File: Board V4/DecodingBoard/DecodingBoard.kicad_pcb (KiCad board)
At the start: 4 copper layers, 0 parts

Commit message: First version of the layout
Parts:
- added C1: 10 μF 6.3V X5R, Capacitor_SMD:C_0805_2012Metric, F.Cu at (109.5, 73.0)
- added C10: 100nF, Capacitor_SMD:C_0402_1005Metric, F.Cu at (116.8, 73.8)
- added C11: 100nF, Capacitor_SMD:C_0402_1005Metric, F.Cu at (119.0, 75.0)
- added C12: 100nF, Capacitor_SMD:C_0402_1005Metric, F.Cu at (119.0, 73.8)
- added C13: 10uF, Capacitor_SMD:C_0603_1608Metric, F.Cu at (117.7, 76.5)
- added C14: 100nF, Capacitor_SMD:C_0402_1005Metric, F.Cu at (110.5, 69.5)
- added C15: 1uF, Capacitor_SMD:C_0402_1005Metric, F.Cu at (109.2, 69.5)
- added C16: 10uF, Capacitor_SMD:C_0603_1608Metric, F.Cu at (126.7, 70.7)
- added C17: 10uF, Capacitor_SMD:C_0603_1608Metric, F.Cu at (123.5, 70.7)
- added C18: 0.01uF, Capacitor_SMD:C_0402_1005Metric, F.Cu at (133.3, 73.2)
- added C19: 10pF, Capacitor_SMD:C_0603_1608Metric, F.Cu at (111.0, 56.0)
- added C2: 220pF, Capacitor_SMD:C_0402_1005Metric, F.Cu at (128.3, 66.7)
- added C20: 10pF, Capacitor_SMD:C_0603_1608Metric, F.Cu at (117.2, 53.0)
- added C21: 100nF, Capacitor_SMD:C_0402_1005Metric, B.Cu at (126.0, 75.2)
- added C22: 100nF, Capacitor_SMD:C_0402_1005Metric, B.Cu at (113.5, 81.4)
- added C23: 100nF, Capacitor_SMD:C_0402_1005Metric, F.Cu at (112.0, 74.2)
- added C24: 100nF, Capacitor_SMD:C_0402_1005Metric, F.Cu at (137.3, 69.8)
- added C25: 4.7uF, Capacitor_SMD:C_0603_1608Metric, F.Cu at (137.3, 68.2)
- added C26: 100nF, Capacitor_SMD:C_0402_1005Metric, F.Cu at (137.5, 76.4)
- added C27: 10uF, Capacitor_SMD:C_0603_1608Metric, F.Cu at (137.5, 77.9)
- added C28: 100nF, Capacitor_SMD:C_0402_1005Metric, F.Cu at (134.8, 69.8)
- added C29: 10uF, Capacitor_SMD:C_0603_1608Metric, F.Cu at (134.3, 68.2)
- added C3: 4.7uF, Capacitor_SMD:C_0603_1608Metric, F.Cu at (114.0, 61.5)
- added C31: 100nF, Capacitor_SMD:C_0402_1005Metric, F.Cu at (131.9, 80.2)
- added C4: 10uF, Capacitor_SMD:C_0603_1608Metric, F.Cu at (112.2, 61.5)
- added C5: 100nF, Capacitor_SMD:C_0402_1005Metric, F.Cu at (118.0, 62.0)
- added C6: 100nF, Capacitor_SMD:C_0402_1005Metric, F.Cu at (115.5, 62.0)
- added C7: 470nF, Capacitor_SMD:C_0402_1005Metric, F.Cu at (119.2, 62.0)
- added C8: 100nF, Capacitor_SMD:C_0402_1005Metric, F.Cu at (116.8, 62.0)
- added C9: 100nF, Capacitor_SMD:C_0402_1005Metric, F.Cu at (116.8, 75.0)
- added D1: IN_S42BT LED, LED_SMD:LED_0402_1005Metric, F.Cu at (122.0, 73.5)
- added D2: IN_S42BT LED, LED_SMD:LED_0402_1005Metric, F.Cu at (103.5, 75.0)
- added D6: IN_S42BT LED, LED_SMD:LED_0402_1005Metric, F.Cu at (129.3, 70.5)
- added H1: MountingHole_Pad, MountingHole:MountingHole_2.2mm_M2_DIN965_Pad, F.Cu at (111.0, 52.0)
- added H2: MountingHole_Pad, MountingHole:MountingHole_2.2mm_M2_DIN965_Pad, F.Cu at (130.3, 87.2)
- added IC1: STM32WBA65CIU6, Footprints:QFN50P700X700X60-49N-D, F.Cu at (115.8, 68.5)
- added IC2: RN4871-V_RM140, Footprints:RN4871VRM140, F.Cu at (106.2, 83.2)
- added IC3: MCP111-195I_TO, Footprints:LR645N3GP013, F.Cu at (102.9, 71.5)
- added J1: UJ20-C-H-G-SMT-1-P16-TR, Footprints:SAMESKY_UJ20-C-H-G-SMT-1-P16-TR, F.Cu at (141.0, 84.1)
- added J2: 2053380002, Footprints:CONN_2053380000-SD_02_MOL, F.Cu at (103.2, 62.2)
- added J4: 5040500491, Footprints:CONN_5040500491_MOL, F.Cu at (125.4, 53.1)
- added J5: Conn_01x06_Pin, Connector_PinHeader_2.54mm:PinHeader_1x06_P2.54mm_Vertical_SMD_Pin1Left, F.Cu at (136.8, 57.6)
- added J6: 5037630491, Footprints:CONN_5037630000-SD_04_MOL, F.Cu at (103.8, 52.8)
- added L2: 2.2uH, Inductor_SMD:L_0805_2012Metric, F.Cu at (110.0, 63.1)
- added R1: 100, Resistor_SMD:R_0402_1005Metric, B.Cu at (122.2, 59.2)
- added R10: 51.1k, Resistor_SMD:R_0402_1005Metric, B.Cu at (134.5, 71.2)
- added R11: 23.7k, Resistor_SMD:R_0402_1005Metric, B.Cu at (136.5, 74.2)
- added R12: 5k, Resistor_SMD:R_0402_1005Metric, B.Cu at (138.0, 74.3)
- added R13: 100, Resistor_SMD:R_0402_1005Metric, F.Cu at (128.8, 68.5)
- added R14: 100, Resistor_SMD:R_0402_1005Metric, B.Cu at (123.3, 73.3)
- added R15: 100, Resistor_SMD:R_0402_1005Metric, B.Cu at (126.1, 77.7)
- added R16: 10k, Resistor_SMD:R_0402_1005Metric, B.Cu at (126.0, 76.5)
- added R17: 100, Resistor_SMD:R_0402_1005Metric, B.Cu at (113.5, 83.9)
- added R18: 4.7k, Resistor_SMD:R_0402_1005Metric, B.Cu at (100.4, 69.8)
- added R19: 330, Resistor_SMD:R_0402_1005Metric, B.Cu at (113.3, 77.5)
- added R2: 100, Resistor_SMD:R_0402_1005Metric, B.Cu at (128.0, 59.5)
- added R3: 4.7k, Resistor_SMD:R_0603_1608Metric, B.Cu at (105.9, 57.2)
- added R4: 4.7k, Resistor_SMD:R_0603_1608Metric, B.Cu at (102.2, 57.2)
- added R5: 5.1k, Resistor_SMD:R_0402_1005Metric, B.Cu at (131.7, 83.4)
- added R6: 5.1k, Resistor_SMD:R_0402_1005Metric, B.Cu at (131.4, 80.2)
- added R7: 86.8k, Resistor_SMD:R_0603_1608Metric, B.Cu at (129.3, 65.0)
- added R8: 23.7k, Resistor_SMD:R_0402_1005Metric, B.Cu at (120.5, 70.4)
- added R9: 5k, Resistor_SMD:R_0402_1005Metric, B.Cu at (137.3, 72.5)
- added SW1: TL3305BF100QG, Footprints:TL3305BF160QG, F.Cu at (124.5, 83.8)
- added SW2: TL3305BF100QG, Footprints:TL3305BF160QG, F.Cu at (117.5, 83.8)
- added TP1: TestPoint, TestPoint:TestPoint_Pad_D1.0mm, F.Cu at (107.8, 76.0)
- added U1: ESDS302DBVR, Footprints:SOT95P280X145-5N, F.Cu at (125.0, 59.9)
- added U2: TPS7A7200RGWT, Footprints:QFN65P500X500X100-21N-D, F.Cu at (124.3, 66.3)
- added U3: USBLC6-2SC6, Package_TO_SOT_SMD:SOT-23-6, F.Cu at (130.4, 83.2)
- added U4: TPS2121RUXR, Footprints:TPS2121RUXR, F.Cu at (136.6, 73.5)
- added XTAL1: CX2016DB32000D0FLJCC, Footprints:CX2016DB32000D0FLJCC, F.Cu at (116.8, 56.2)
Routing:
- net GND: track 0.00 -> 14.0 mm, vias 0 -> 14

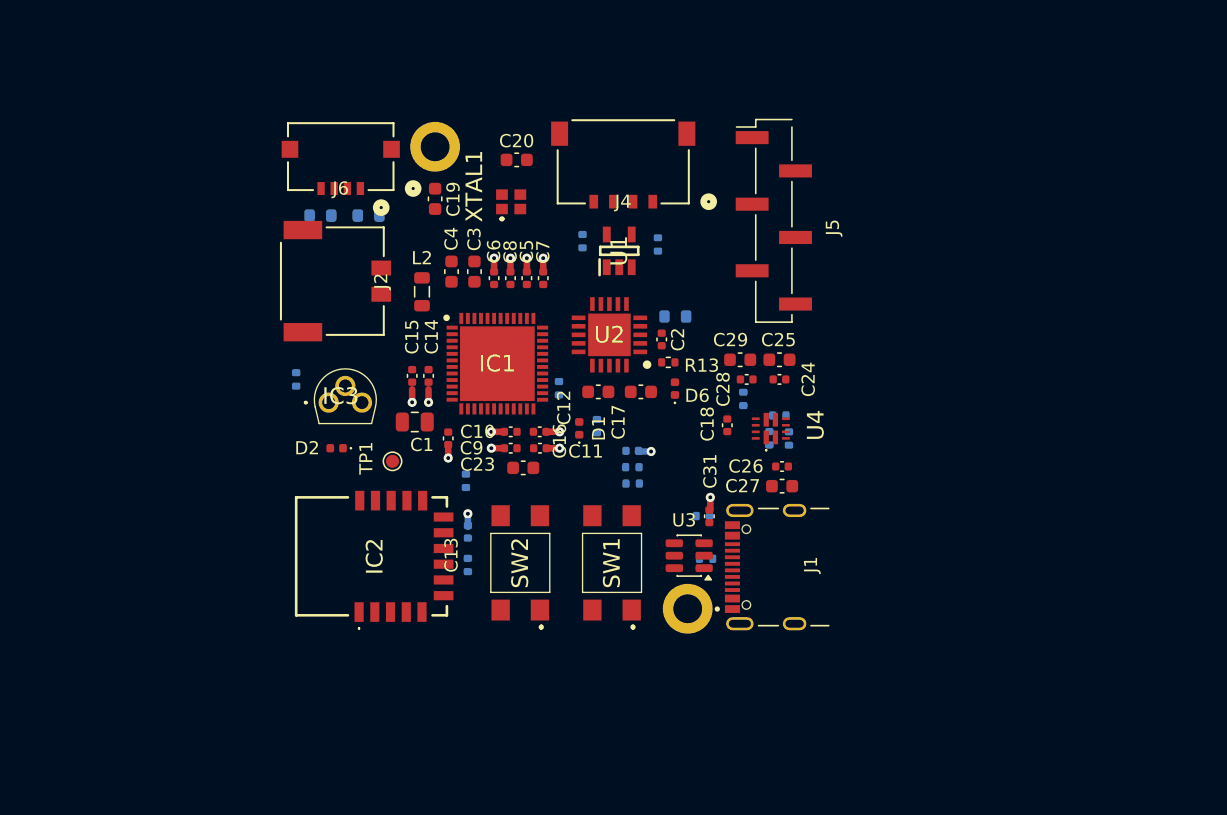
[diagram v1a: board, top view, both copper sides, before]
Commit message: progress on the layout
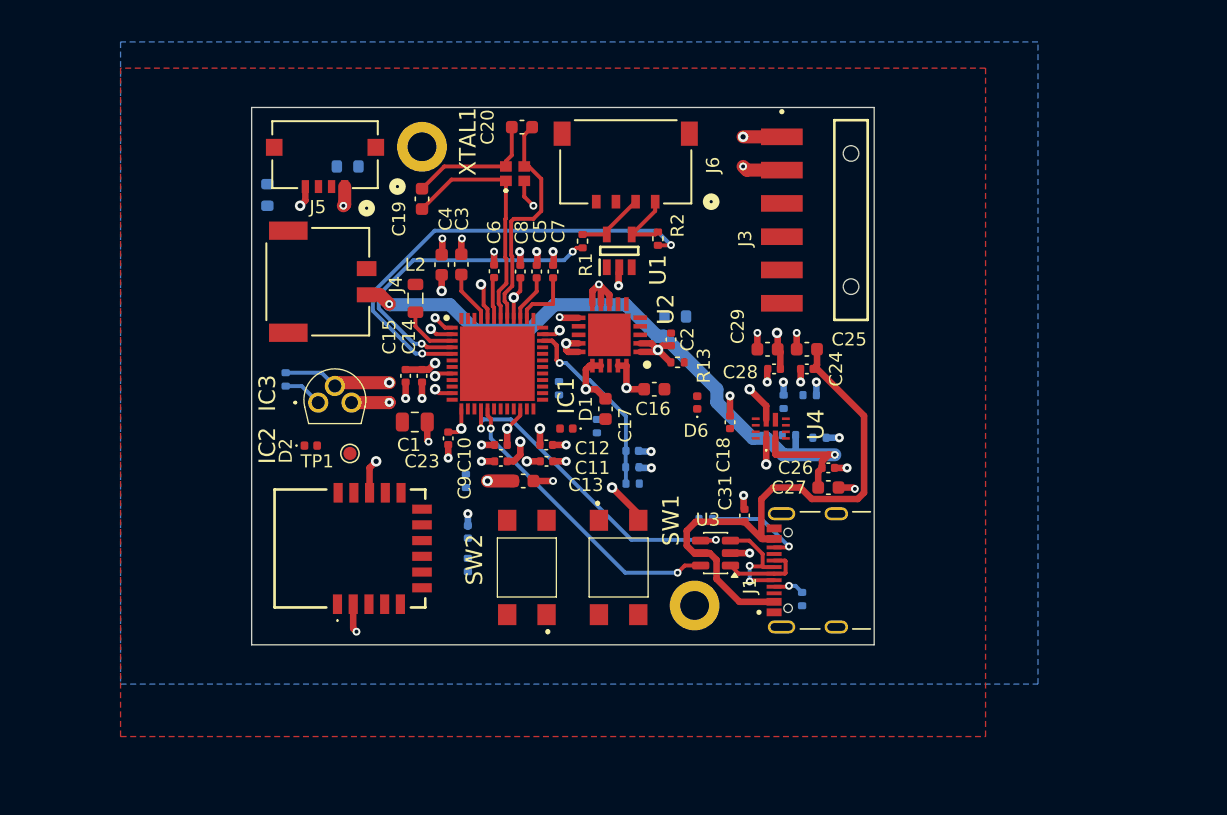
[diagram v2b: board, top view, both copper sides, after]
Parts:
- removed J2: 2053380002, Footprints:CONN_2053380000-SD_02_MOL
- added J3: TSM-106-02-T-SH-LC, Footprints:SAMTEC_TSM-106-02-T-SH-LC, F.Cu at (142.7, 57.6)
- J4: value 5040500491 -> 2053380004; footprint Footprints:CONN_5040500491_MOL -> Footprints:CONN_2053380000-SD_02_MOL
- J5: value Conn_01x06_Pin -> 5037630691; footprint Connector_PinHeader_2.54mm:PinHeader_1x06_P2.54mm_Vertical_SMD_Pin1Left -> Footprints:CONN_5037630000-SD_04_MOL
- J6: value 5037630491 -> 5040500691; footprint Footprints:CONN_5037630000-SD_04_MOL -> Footprints:CONN_5040500491_MOL
- R1, R2: moved to F.Cu
- moved J5 34.6 mm to (102.6, 52.6)
- moved J4 25.0 mm to (102.0, 62.3), turned to 90 degrees
- moved J6 21.7 mm to (125.5, 53.1)
- moved R5 7.94 mm to (139.0, 86.5), turned to -90 degrees
- moved R3 7.88 mm to (98.2, 55.7), turned to 90 degrees
- moved R4 4.29 mm to (104.3, 53.5), turned to 180 degrees
- moved C26 3.53 mm to (141.0, 76.5)
- moved C27 3.53 mm to (141.0, 78.0)
- moved TP1 3.30 mm to (104.5, 75.4)
- moved J1 3.19 mm to (144.2, 84.3)
- moved R10 3.08 mm to (137.6, 71.5)
- moved R9 2.79 mm to (139.6, 71.0)
- moved C31 2.69 mm to (134.6, 80.1)
- moved C20 2.53 mm to (117.6, 50.5)
- moved R12 2.33 mm to (140.3, 74.2), turned to 0 degrees
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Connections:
- J4 pad 1: /USART1_RX_CONN -> GND
- J4 pad 2: /USART1_TX_CONN -> /Power
- J5 pad 1: +3.3V -> GND
- J5 pad 2: GND -> /I2C/I2C_SCL
- J5 pad 3: /SWD_NRST -> /I2C/I2C_SDA
- J5 pad 4: /SWDCLK -> +5V
- J5 pad 5: /SWDIO -> GND
- J5 pad 6: /SWD_TRACES -> GND
- J6 pad 1: GND -> /USART1_RX_CONN
- J6 pad 2: /I2C/I2C_SCL -> /USART1_TX_CONN
- J6 pad 3: /I2C/I2C_SDA -> GND
- J6 pad 4: +5V -> GND
- J6 pad 5: (no net) -> GND
- J6 pad 6: (no net) -> GND
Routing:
- net +3.3V: track 0.00 -> 54.7 mm, vias 0 -> 20
- net /Power: track 0.00 -> 53.2 mm, vias 0 -> 2
- net GND: track 14.0 -> 64.0 mm, vias 14 -> 39
- net /Power switching and voltage adaptation/from USB-C: track 0.00 -> 43.5 mm
- net /USART1_RX: track 0.00 -> 35.0 mm, vias 0 -> 2
- net /USB-C circuit/D-: track 0.00 -> 25.0 mm, vias 0 -> 2
- net /USART1_TX: track 0.00 -> 24.9 mm, vias 0 -> 2
- net /USB-C circuit/D+: track 0.00 -> 22.8 mm, vias 0 -> 2
- net /OSC_IN: track 0.00 -> 18.3 mm
- net /OSC_OUT: track 0.00 -> 17.8 mm
- net +5V: track 0.00 -> 16.5 mm, vias 0 -> 6
- net /BOOT0: track 0.00 -> 14.6 mm, vias 0 -> 1
- net /VDD11: track 0.00 -> 10.8 mm
- net /USB-C circuit/USB_D-: track 0.00 -> 8.84 mm, vias 0 -> 2
- net /USB-C circuit/USB_CC2: track 0.00 -> 7.87 mm, vias 0 -> 1
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- added copper zone on In2.Cu, net +3.3V
- added copper zone on In2.Cu, net +5V
- added copper zone on B.Cu, net GND
- added copper zone on F.Cu, net GND
- added copper zone on In1.Cu, net GND
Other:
- board outline added: 47.5 x 41 mm
- rule pad_to_mask_clearance: 0.08 -> 0

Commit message: complete first PCB layout
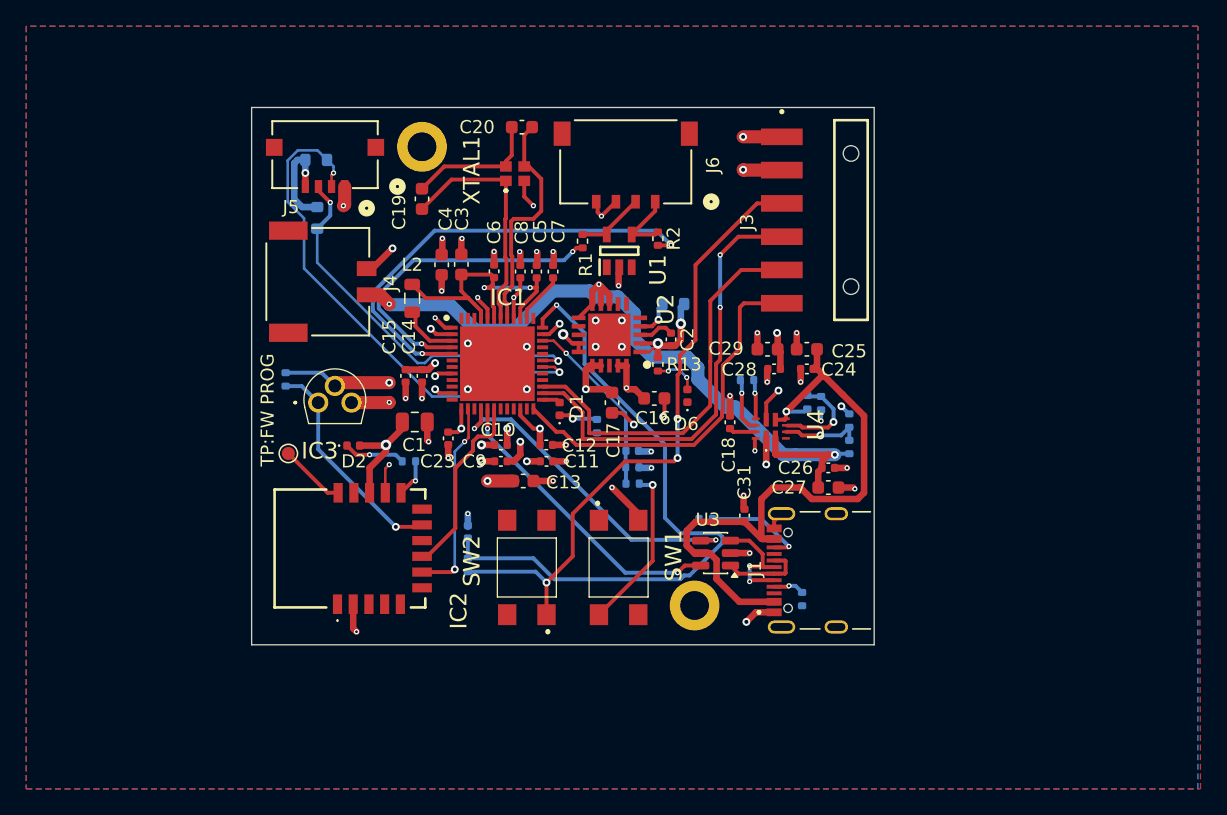
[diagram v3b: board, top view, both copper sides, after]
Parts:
- moved R8 19.0 mm to (139.4, 71.5), turned to 90 degrees
- moved TP1 4.70 mm to (99.8, 75.4)
- moved R11 4.69 mm to (142.6, 74.9), turned to 90 degrees
- moved R19 4.60 mm to (109.0, 76.0), turned to 180 degrees
- moved R3 4.18 mm to (102.0, 57.4), turned to -90 degrees
- moved D2 3.25 mm to (104.8, 74.8)
- moved R10 3.25 mm to (134.8, 69.8), turned to 0 degrees
- moved R12 2.62 mm to (142.6, 72.9), turned to 90 degrees
- moved R4 2.45 mm to (101.9, 53.0), turned to 0 degrees
- moved D1 1.59 mm to (120.5, 72.0), turned to 90 degrees
- moved R13 1.51 mm to (128.0, 68.6), turned to -90 degrees
- moved R9 1.06 mm to (140.4, 71.6), turned to -90 degrees
- moved R7 0.96 mm to (129.2, 64.0)
- moved D6 0.91 mm to (130.2, 71.0)
- moved C16 0.70 mm to (127.7, 71.2)
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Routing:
- net Net-(IC1-NRST): track 0.00 -> 50.0 mm, vias 0 -> 1
- net /SWD_NRST: track 0.00 -> 48.5 mm, vias 0 -> 3
- net /I2C/I2C_SCL: track 0.00 -> 40.4 mm, vias 0 -> 2
- net /SWDCLK: track 0.00 -> 34.3 mm, vias 0 -> 2
- net /SWDIO: track 0.00 -> 30.6 mm
- net /SWD_TRACES: track 0.00 -> 29.9 mm
- net /I2C/I2C_SDA: track 0.00 -> 29.9 mm, vias 0 -> 2
- net GND: track 64.0 -> 81.5 mm, vias 39 -> 53
- net /USART2_RX_BLE: track 0.00 -> 15.3 mm, vias 0 -> 2
- net /USART2_RX_MCU: track 0.00 -> 14.3 mm
- net Net-(IC2-RST_N): track 3.00 -> 17.0 mm, vias 0 -> 1
- net Net-(R15-Pad1): track 0.00 -> 12.7 mm, vias 0 -> 1
- net /VDD11: track 10.8 -> 22.8 mm, vias 0 -> 2
- net +3.3V: track 54.7 -> 63.9 mm, vias 20 -> 21
- net /Power switching and voltage adaptation/from USB-C: track 43.5 -> 50.6 mm, vias 0 -> 1
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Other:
- board text added: "TP:FW PROG"
